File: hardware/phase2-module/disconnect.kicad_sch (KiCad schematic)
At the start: 18 parts, among them Q10 CSD18540Q5B, Q11 CSD18540Q5B, Q3 CSD18540Q5B, Q4 CSD18540Q5B, Q7 2N7002, Q9 2N7002, U6 LTC7004, U7 TLV7011DCK

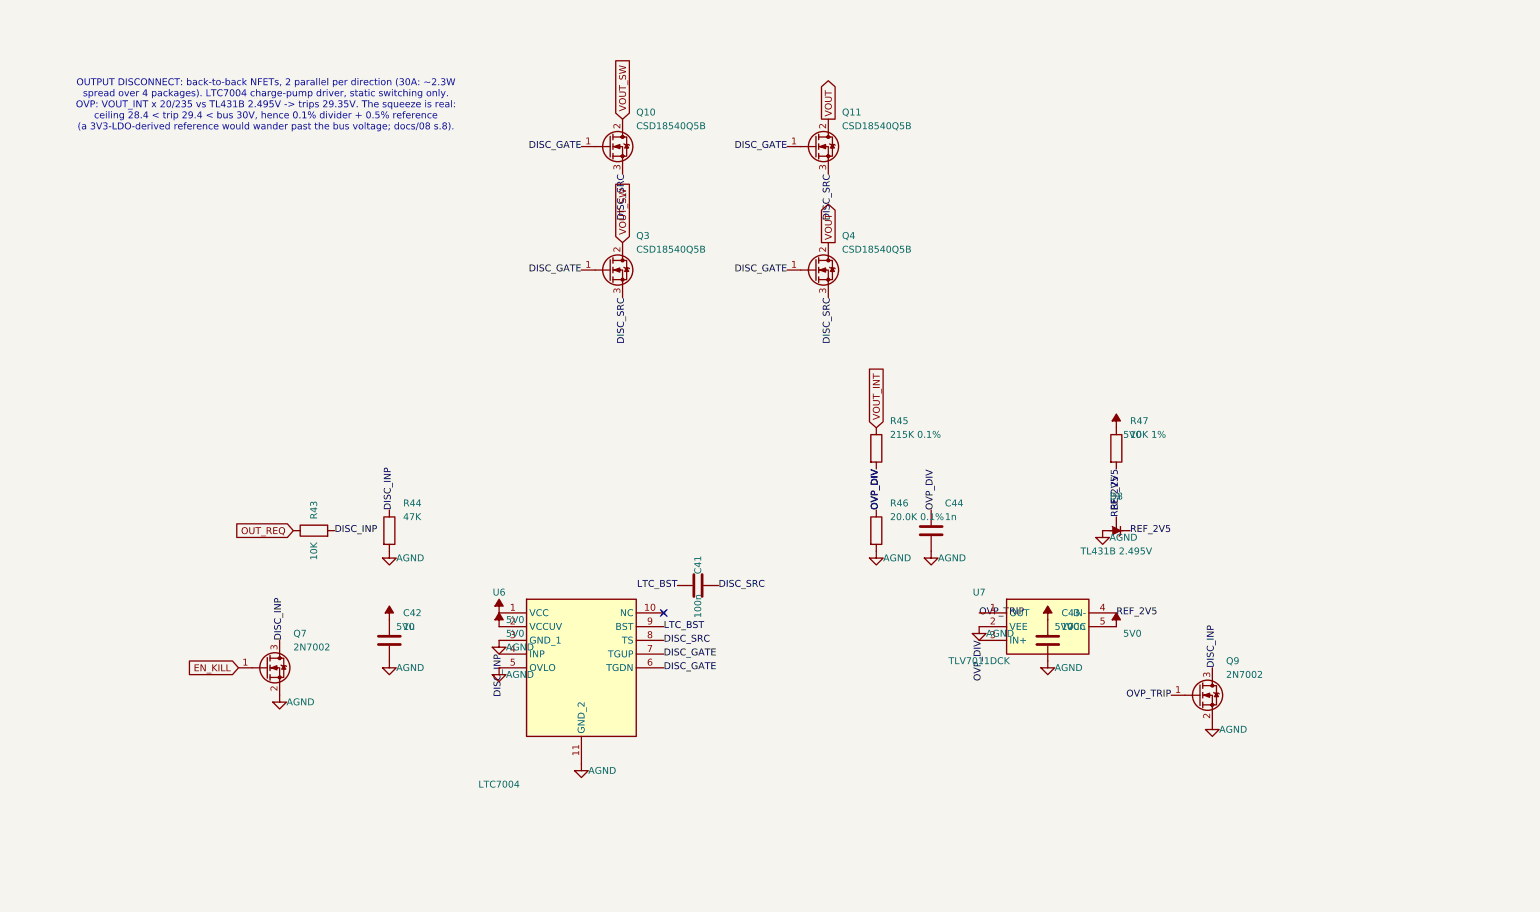
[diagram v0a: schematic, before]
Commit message: Add autosaved schematic files for power stage and auxiliary rails in phase2-module
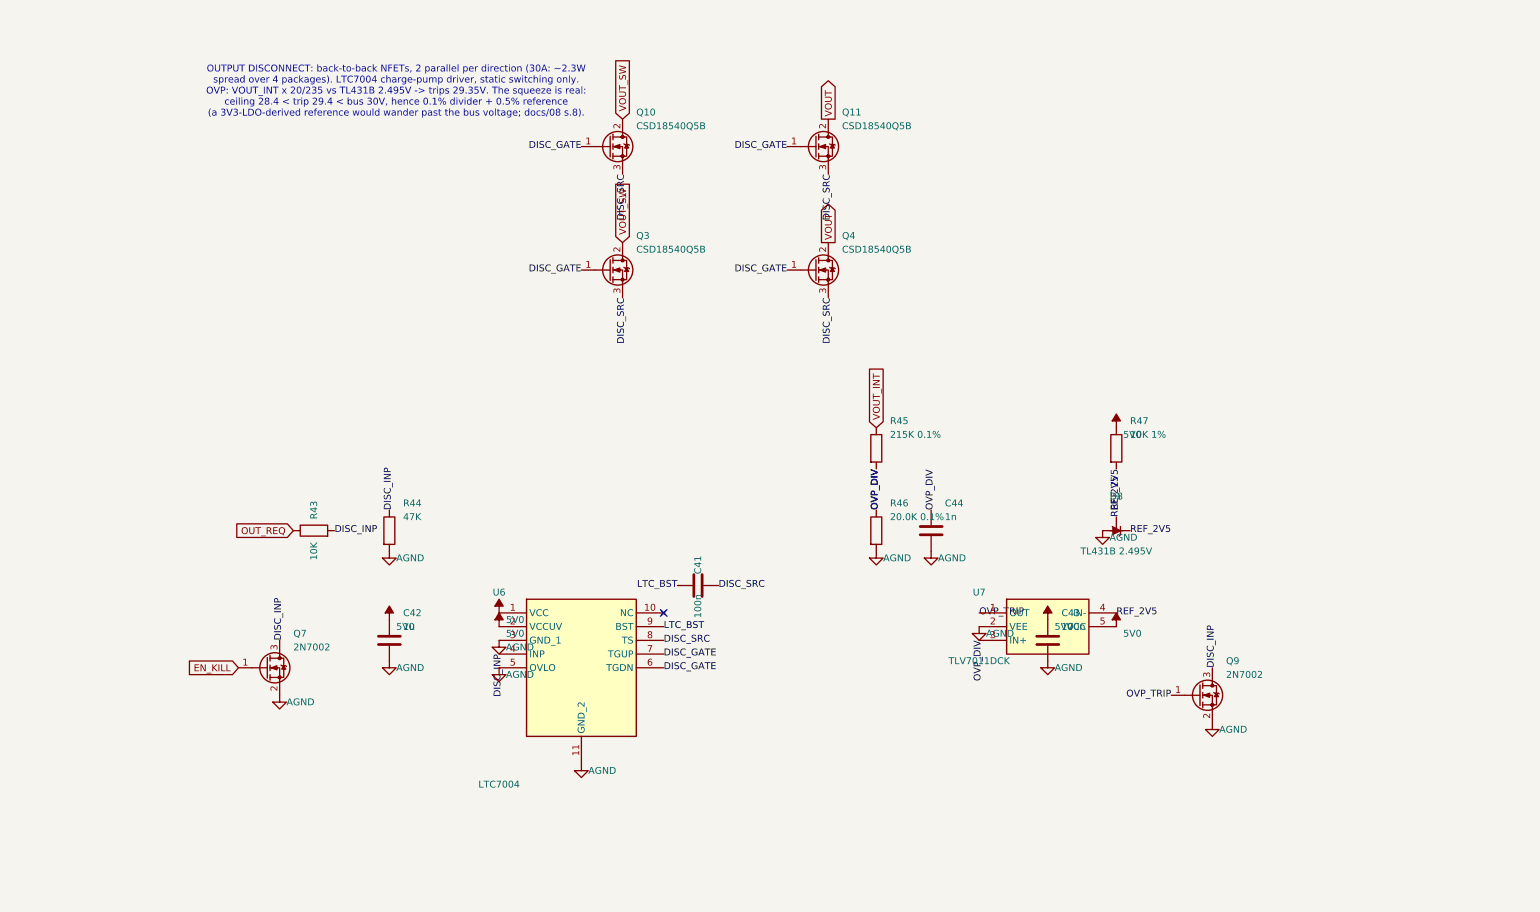
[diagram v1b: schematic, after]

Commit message: Refactor code structure for improved readability and maintainability
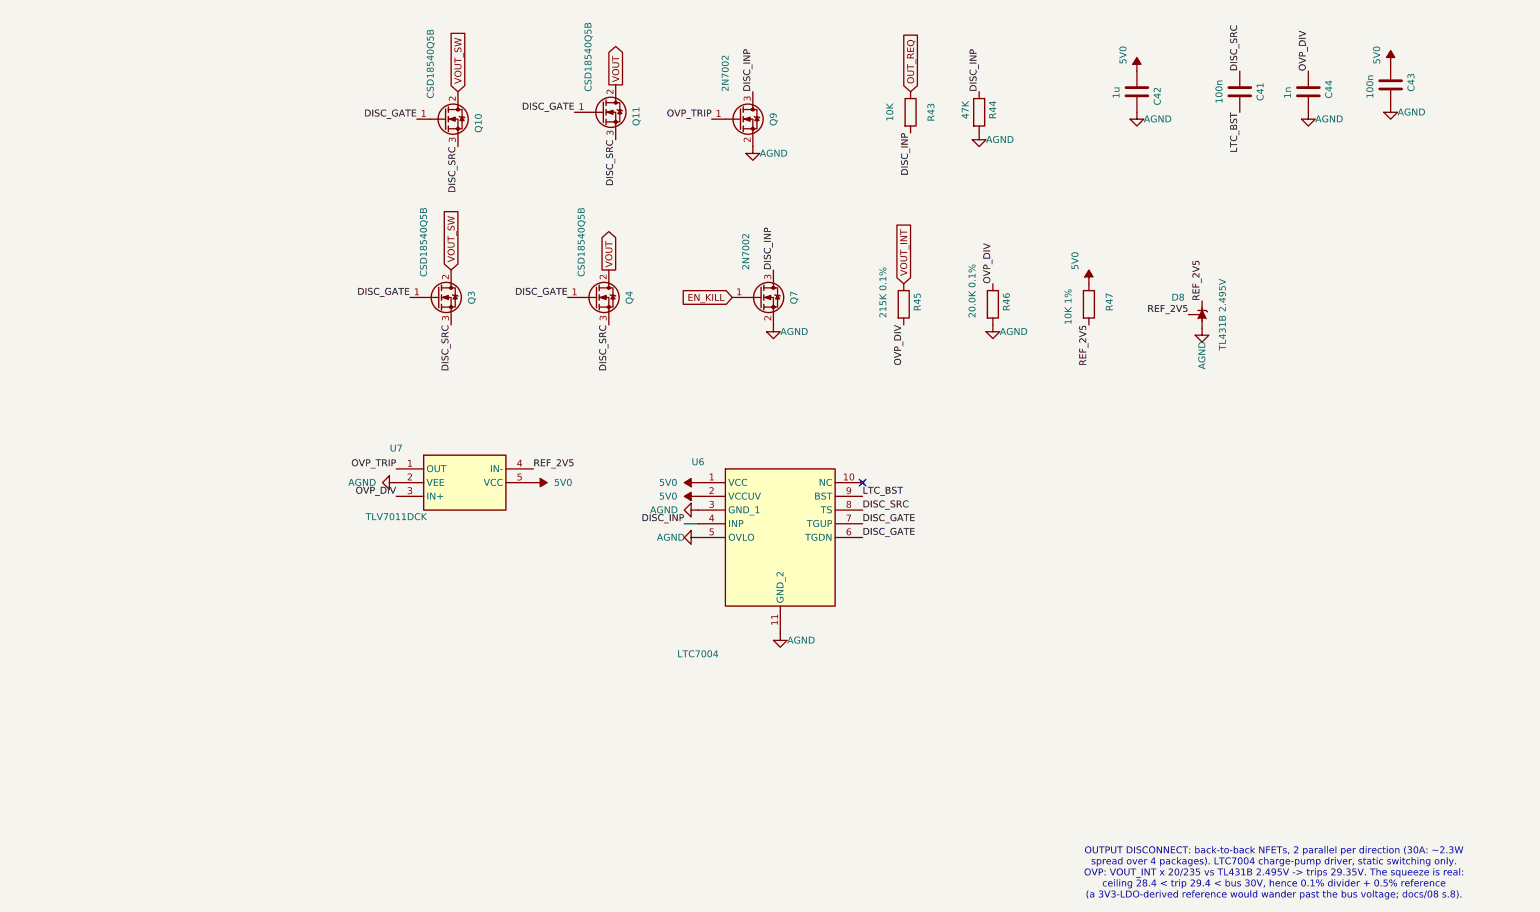
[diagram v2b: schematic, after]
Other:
- moved on the sheet: C41, C42, C43, C44, D8, Q10, Q11, Q3, Q4, Q7, Q9, R43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
